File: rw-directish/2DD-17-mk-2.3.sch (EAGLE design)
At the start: 28 parts, among them J1 AVR_SPI_PRG_6PTH, U1 MPS28164, U2 ATTINY25-20MU, U3 INA190RSW, U4 TLV30028DCK

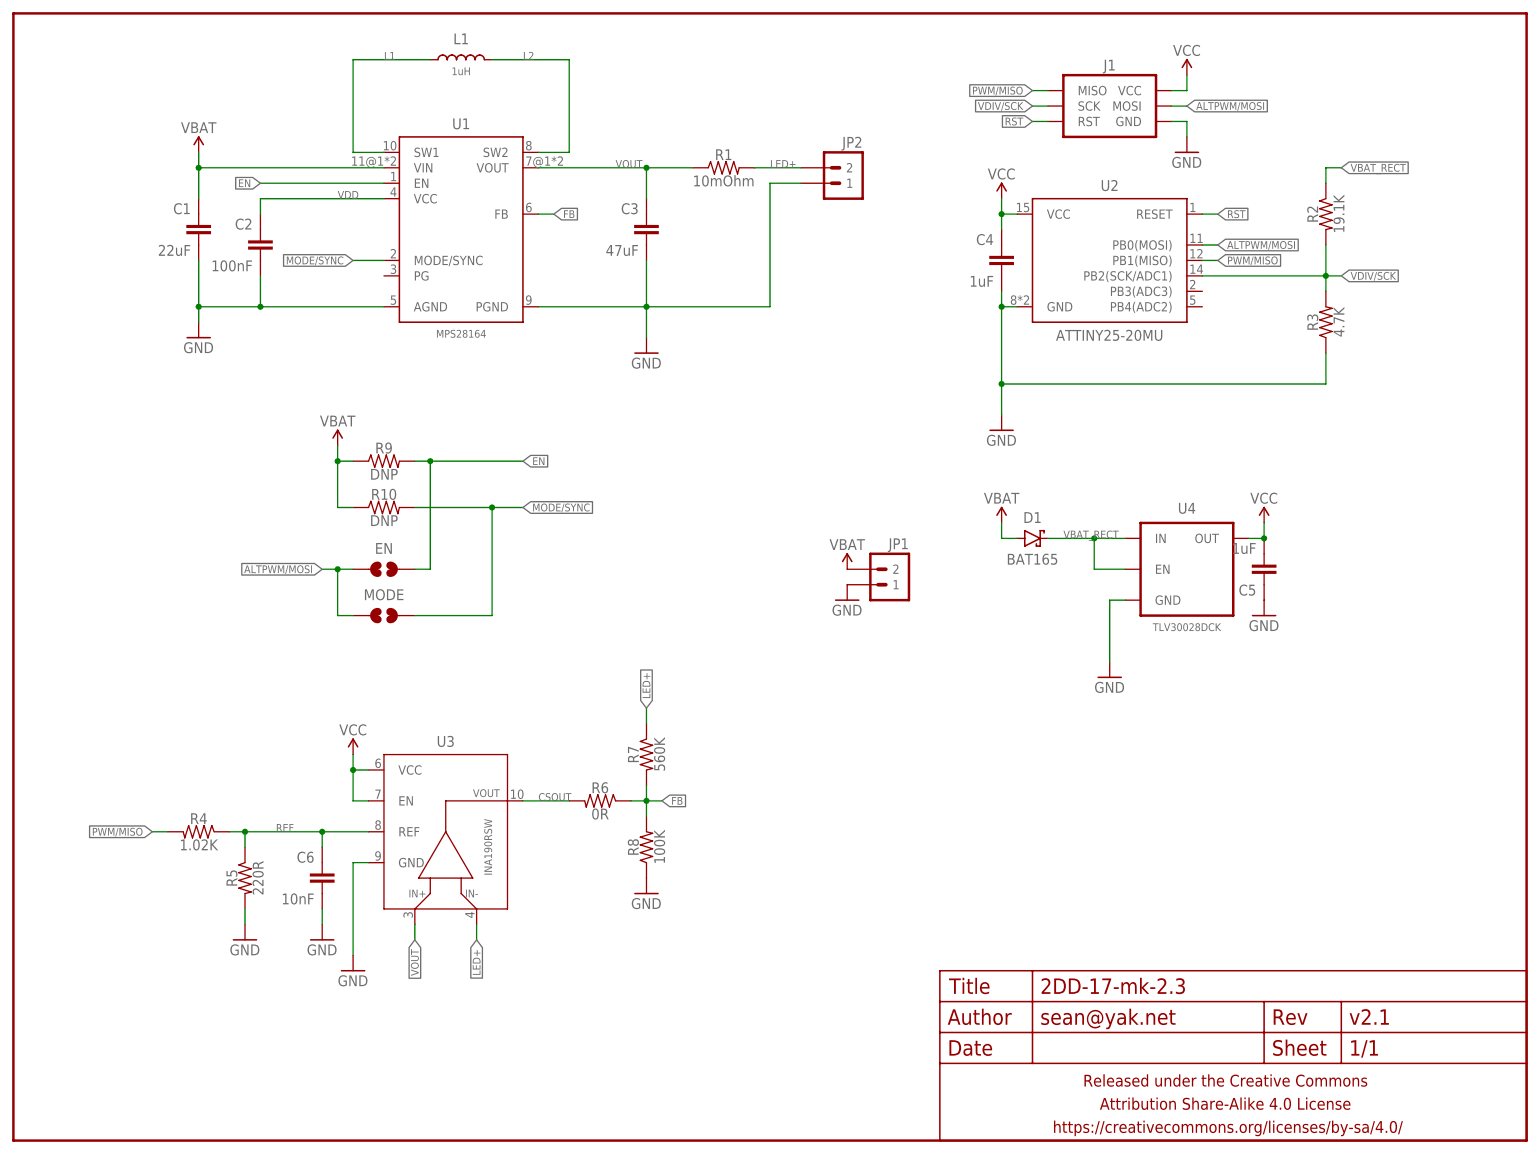
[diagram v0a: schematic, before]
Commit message: wip buck boost
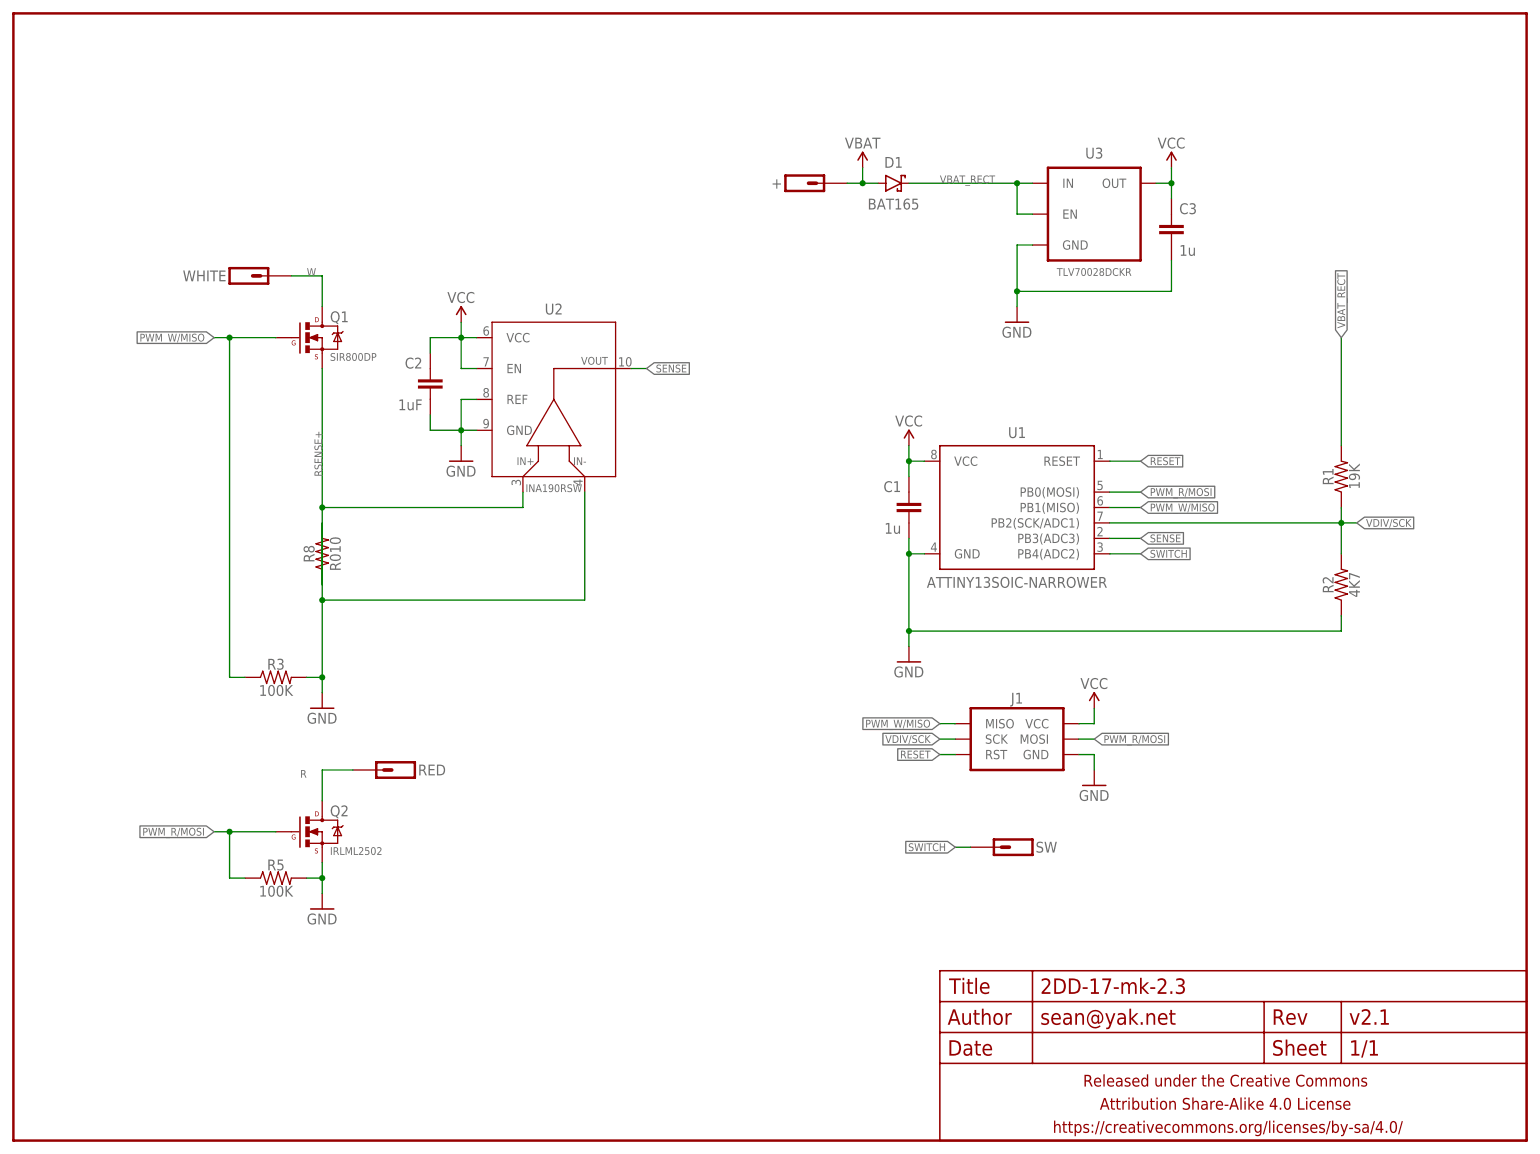
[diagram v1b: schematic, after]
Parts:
- removed C4, C5: 1uF, a_parts:CAPACITOR-CERAMICC0402
- removed C6: 10nF, a_parts:CAPACITOR-CERAMICC0402
- removed EN, MODE: JUMPER-PAD-2-NOYES_SILK, a_parts:JUMPER-PAD-2-NOYES_SILK
- removed JP1, JP2: M021X02_NO_SILK, a_parts:M021X02_NO_SILK
- removed L1: 1uH, a_parts:INDUCTORXAL60XX
- removed R10, R9: DNP, a_parts:RESISTORR0402
- removed R4: 1.02K, a_parts:RESISTORR0402
- removed R6: 0R, a_parts:RESISTORR0402
- removed R7: 560K, a_parts:RESISTORR0402
- removed U4: TLV30028DCK, a_parts:V_REG_ENTLV700XXDCR
- added +: M01PTH-1MM-CIR-NS, a_parts:M01PTH-1MM-CIR-NS
- added Q1: SIR800DP, a_parts:MOSFET-NCHANNELPSMN4R0-30YLD
- added Q2: IRLML2502, a_parts:MOSFET-NCHANNELIRLML2502
- added RED, SW, WHITE: M01SMD-1.25MM-DIA, a_parts:M01SMD-1.25MM-DIA
- C1: value 22uF -> 1u; device a_parts:CAPACITOR-CERAMICC1206 -> a_parts:CAPACITOR-CERAMICC0402
- C2: value 100nF -> 1uF
- C3: value 47uF -> 1u; device a_parts:CAPACITOR-CERAMICC1206 -> a_parts:CAPACITOR-CERAMICC0402
- J1: value AVR_SPI_PRG_6PTH -> AVR_SPI_PRG_6SMD-1.27MM; device a_parts:AVR_SPI_PRG_6PTH -> a_parts:AVR_SPI_PRG_6SMD-1.27MM
- R1: value 10mOhm -> 19K; device a_parts:RESISTORR1206 -> a_parts:RESISTORR0402
- R2: value 19.1K -> 4K7
- R3: value 4.7K -> 100K
- R5: value 220R -> 100K
- R8: value 100K -> R010; device a_parts:RESISTORR0402 -> a_parts:RESISTORR1206
- U1: value MPS28164 -> ATTINY13SOIC-NARROWER; device a_parts:MPS28164 -> a_parts:ATTINY13SOIC-NARROWER
- U2: value ATTINY25-20MU -> INA190RSW; device a_parts:ATTINY45TINY85-20-QFN -> a_parts:INA190RSW
- U3: value INA190RSW -> TLV70028DCKR; device a_parts:INA190RSW -> a_parts:V_REG_ENTLV700XXDCR
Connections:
- removed net ALTPWM/MOSI: EN.1, J1.MOSI, MODE.1, U2.PB0(MOSI)
- removed net CSOUT: R6.2, U3.OUT
- removed net EN: EN.2, R9.2, U1.EN
- removed net FB: R6.1, R7.2, R8.2, U1.FB
- removed net L1: L1.1, U1.SW1
- removed net L2: L1.2, U1.SW2
- removed net LED+: JP2.2, R1.2, R7.1, U3.VIN-
- removed net MODE/SYNC: MODE.2, R10.2, U1.MODE/SYNC
- removed net PWM/MISO: J1.MISO, R4.2, U2.PB1(MISO)
- removed net REF: C6.1, R4.1, R5.1, U3.REF
- removed net RST: J1.RST, U2.RESET
- removed net VDD: C2.1, U1.VCC
- removed net VOUT: C3.1, R1.1, U1.VOUT, U3.VIN+
- new net PWM_R/MOSI: J1.MOSI, Q2.G, R5.1, U1.PB0(MOSI)
- new net PWM_W/MISO: J1.MISO, Q1.G, R3.1, U1.PB1(MISO)
- new net R: Q2.D, RED.1
- new net RESET: J1.RST, U1.RESET
- new net RSENSE+: Q1.S, R8.1, U2.VIN+
- new net SENSE: U1.PB3(ADC3), U2.OUT
- new net SWITCH: SW.1, U1.PB4(ADC2)
- new net W: Q1.D, WHITE.1
- net GND: now also Q2.S, R2.1, R3.2, R8.2, U1.GND, U2.REF, U2.VIN-; no longer C4.2, C5.1, C6.2, JP1.1, JP2.1, R3.1, R8.1, U1.AGND, U1.PGND, U4.GND
- net VBAT: now also +.1; no longer C1.1, JP1.2, R10.1, R9.1, U1.VIN
- net VBAT_RECT: now also R1.2, U3.EN, U3.IN; no longer R2.1, U4.EN, U4.IN
- net VCC: now also C1.1, C2.1, C3.1, U1.VCC, U2.EN, U3.OUT; no longer C4.1, C5.2, U3.EN, U3.VCC, U4.OUT
- net VDIV/SCK: now also R1.1, U1.PB2(SCK/ADC1); no longer R3.2, U2.PB2(SCK/ADC1)
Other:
- note removed: "For 1.8V operation, U2 = ATTINY{2,4,8}5-10MU U4 = TLV70018DCK"
- note removed: "For 2.8V operation, U2 = ATTINY{2,4,8}5-20MU U4 = TLV70028DCK"
- moved on the sheet: C1, C2, C3, D1, J1, R1, R2, R3, R5, R8
